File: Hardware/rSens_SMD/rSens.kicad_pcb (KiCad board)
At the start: 2 copper layers, 48.5 x 24.9 mm, 18 parts, among them U2 MCP6244

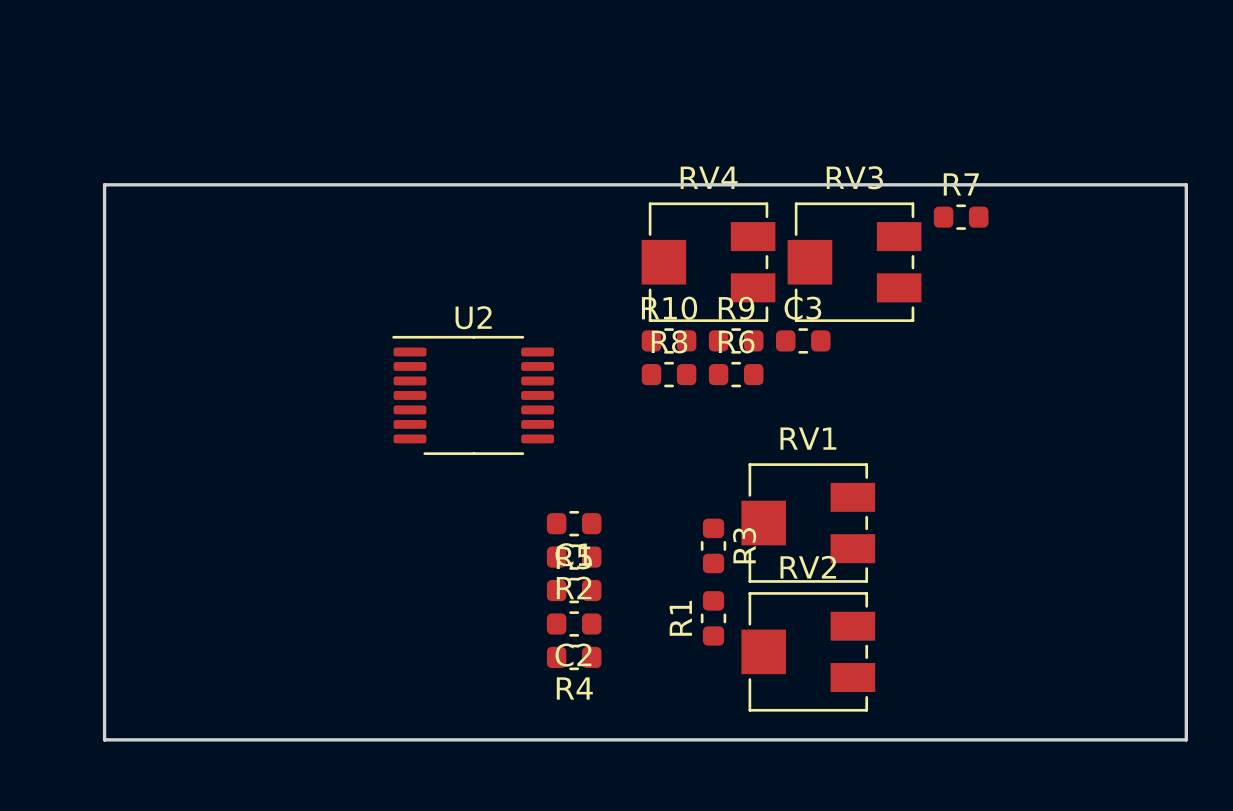
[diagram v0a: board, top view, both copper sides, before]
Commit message: Routing in progress
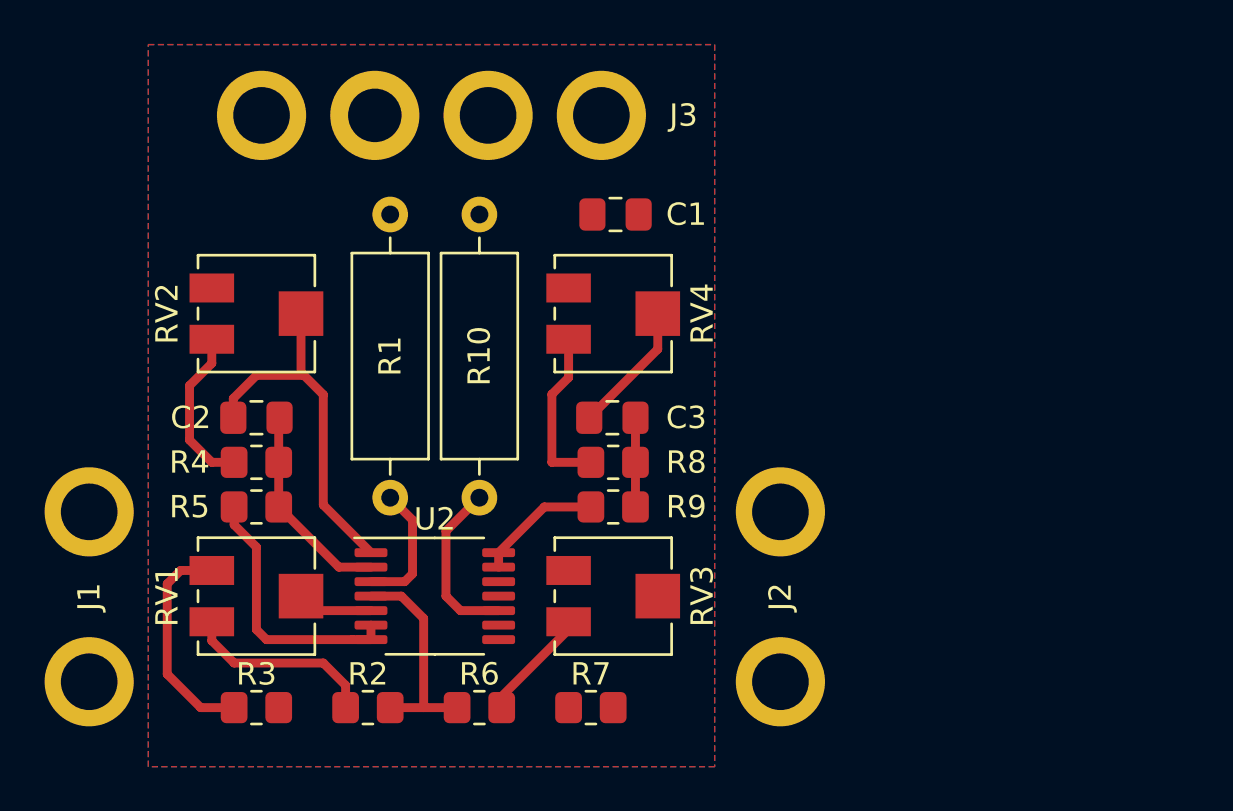
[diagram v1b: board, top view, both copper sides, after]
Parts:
- added J1: Conn_01x02, rSens:rSens_Pad_1x02, F.Cu at (127.8, 101.0)
- added J2: Conn_01x02, rSens:rSens_Pad_1x02, F.Cu at (158.8, 101.0)
- added J3: Conn_01x04, rSens:rSens_Pad_1x04, F.Cu at (140.6, 79.4)
- C1, C2, C3: footprint Capacitor_SMD:C_0603_1608Metric -> Capacitor_SMD:C_0805_2012Metric_Pad1.18x1.45mm_HandSolder
- R1, R10: footprint Resistor_SMD:R_0603_1608Metric -> Resistor_THT:R_Axial_DIN0309_L9.0mm_D3.2mm_P12.70mm_Horizontal
- R2, R3, R4, R5, R6, R7, R8, R9: footprint Resistor_SMD:R_0603_1608Metric -> Resistor_SMD:R_0805_2012Metric_Pad1.20x1.40mm_HandSolder
- moved RV2 29.0 mm to (135.3, 88.3), turned to 180 degrees
- moved R7 27.6 mm to (150.3, 106.0), turned to 180 degrees
- moved RV1 25.0 mm to (135.3, 101.0), turned to 180 degrees
- moved R3 21.7 mm to (135.3, 106.0), turned to 0 degrees
- moved R6 18.9 mm to (145.3, 106.0)
- moved RV3 18.5 mm to (151.3, 101.0), turned to 180 degrees
- moved C2 17.0 mm to (135.3, 93.0), turned to 0 degrees
- moved R4 16.7 mm to (135.3, 95.0), turned to 0 degrees
- moved R1 15.5 mm to (141.3, 96.6)
- moved R5 14.7 mm to (135.3, 97.0), turned to 180 degrees
- moved C1 14.0 mm to (151.4, 83.9)
- moved R2 11.5 mm to (140.3, 106.0)
- moved R10 11.0 mm to (145.3, 96.6), turned to 90 degrees
- moved R9 9.27 mm to (151.3, 97.0), turned to 180 degrees
- moved C3 9.23 mm to (151.3, 93.0)
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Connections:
- R10 pad 1: Net-(C3-Pad2) -> SENSOR_INPUT_B
- R10 pad 2: Net-(R10-Pad2) -> GND
- R8 pad 1: SENSOR_INPUT_B -> Net-(R8-Pad1)
- R8 pad 2: GND -> Net-(C3-Pad2)
- R9 pad 1: Net-(R9-Pad1) -> Net-(C3-Pad2)
- R9 pad 2: Net-(C3-Pad2) -> Net-(R9-Pad2)
- RV4 pad 1: Net-(R9-Pad1) -> Net-(R8-Pad1)
- U2 pad 13: Net-(R10-Pad2) -> Net-(R9-Pad2)
- U2 pad 14: Net-(R10-Pad2) -> Net-(R9-Pad2)
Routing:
- net VOLTAGE_OUTPUT_A: track 0.00 -> 16.5 mm
- net Net-(R5-Pad2): track 0.00 -> 11.9 mm
- net Net-(R3-Pad1): track 0.00 -> 9.92 mm
- net VCC: track 0.00 -> 9.78 mm
- net Net-(C2-Pad2): track 0.00 -> 9.27 mm
- net Net-(R2-Pad2): track 0.00 -> 8.68 mm
- net SENSOR_INPUT_B: track 0.00 -> 7.67 mm
- net Net-(R4-Pad1): track 0.00 -> 7.35 mm
- net Net-(R8-Pad1): track 0.00 -> 6.91 mm
- net SENSOR_INPUT_A: track 0.00 -> 5.84 mm
- net Net-(R9-Pad2): track 0.00 -> 5.64 mm
- net VOLTAGE_OUTPUT_B: track 0.00 -> 5.27 mm
- net Net-(R6-Pad2): track 0.00 -> 5.09 mm
- net Net-(C3-Pad2): track 0.00 -> 4.00 mm
- net Net-(RV1-Pad2): track 0.00 -> 3.41 mm
- added copper zone on F.Cu, net GND
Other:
- board outline removed
- net class Default: trace_width 1 -> 0.4
